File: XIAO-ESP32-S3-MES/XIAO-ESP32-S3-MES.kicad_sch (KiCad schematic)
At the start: 11 parts, among them J1 Conn_01x04_Socket, J2 Conn_01x02_Socket, J3 Conn_01x04_Socket, U2 XIAO-ESP32-S3-SMD

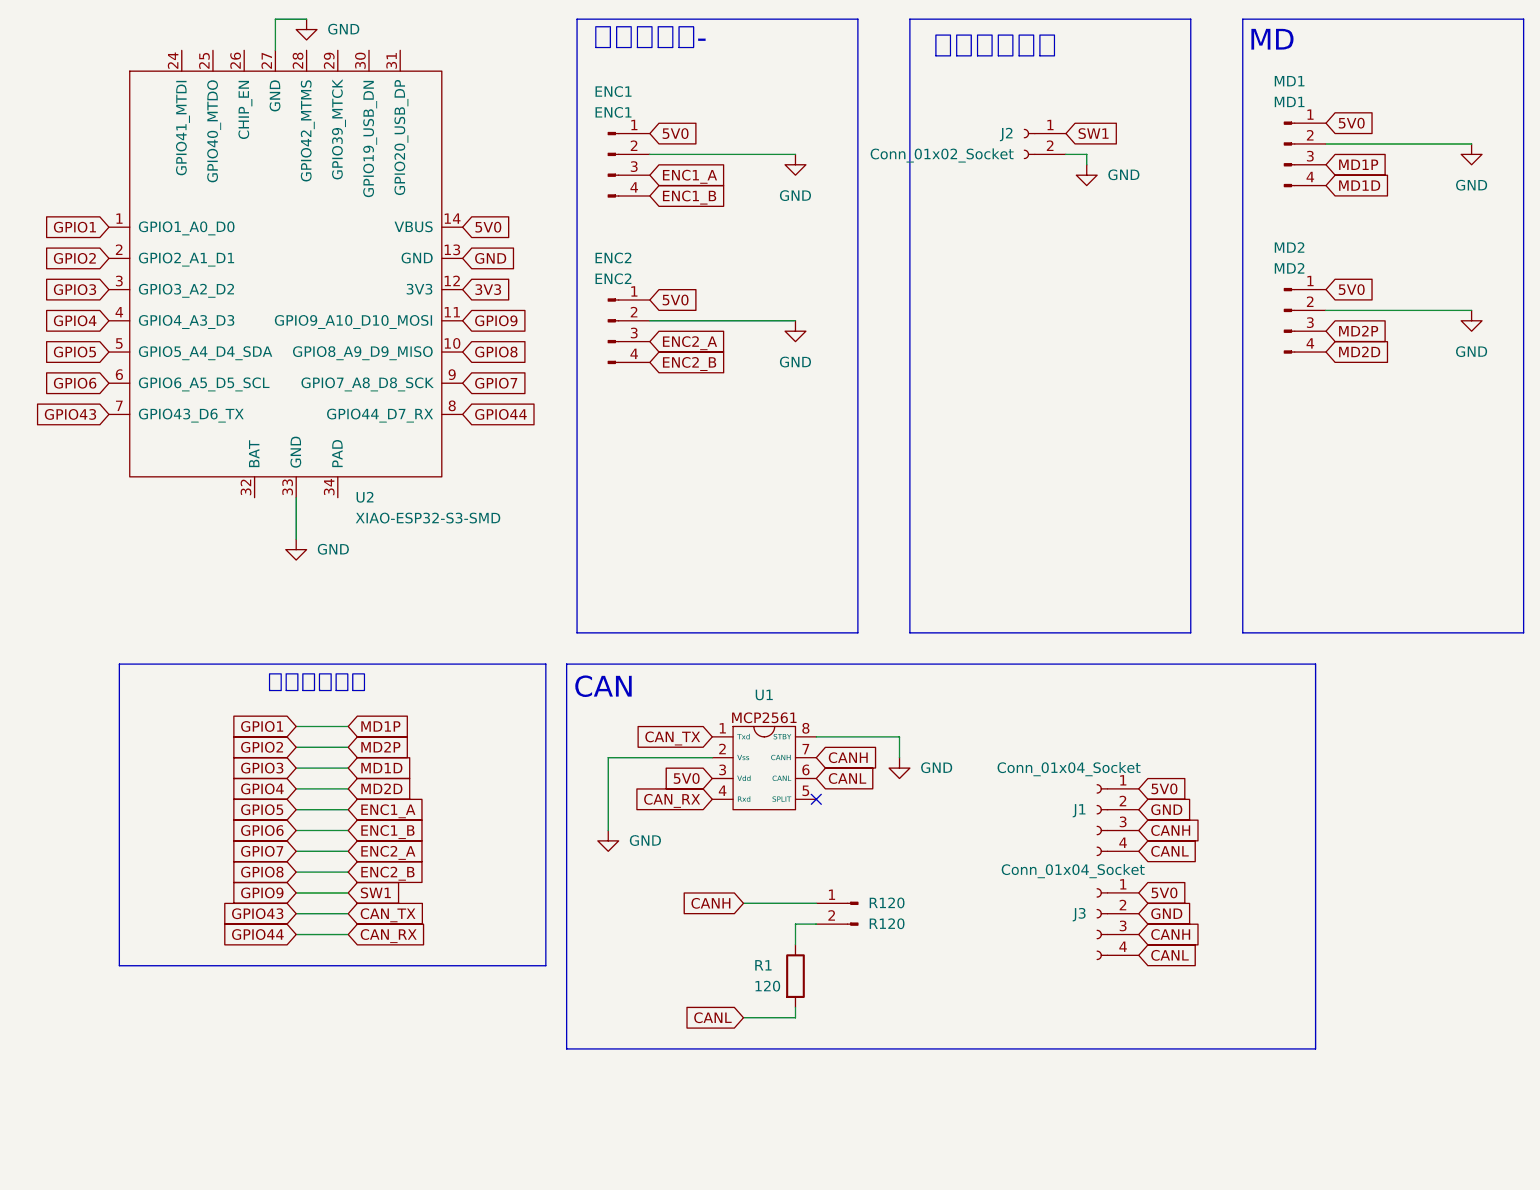
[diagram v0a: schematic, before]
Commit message: 汎用性重視
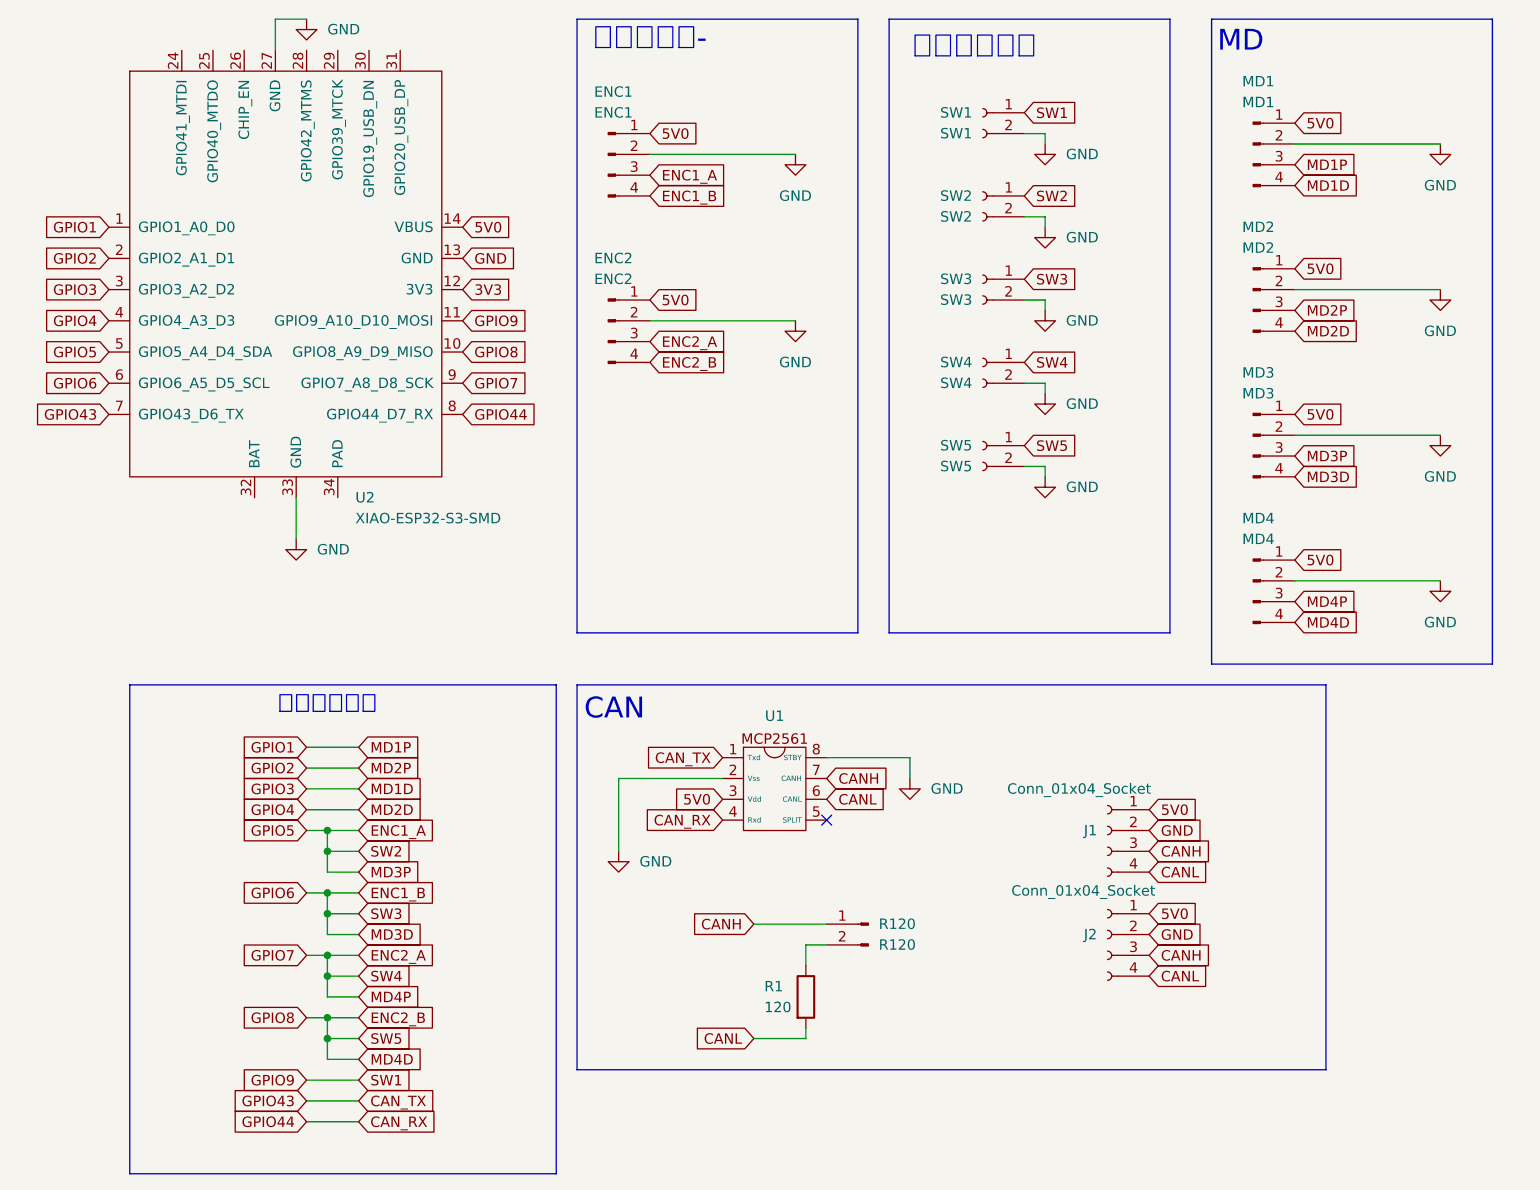
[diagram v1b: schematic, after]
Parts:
- added MD3: MD3, Connector_JST:JST_XH_B4B-XH-A_1x04_P2.50mm_Vertical, symbol Connector:Conn_01x04_Pin
- added MD4: MD4, Connector_JST:JST_XH_B4B-XH-A_1x04_P2.50mm_Vertical, symbol Connector:Conn_01x04_Pin
- added SW2: SW2, Connector_JST:JST_XH_B2B-XH-A_1x02_P2.50mm_Vertical, symbol Connector:Conn_01x02_Socket
- added SW3: SW3, Connector_JST:JST_XH_B2B-XH-A_1x02_P2.50mm_Vertical, symbol Connector:Conn_01x02_Socket
- added SW4: SW4, Connector_JST:JST_XH_B2B-XH-A_1x02_P2.50mm_Vertical, symbol Connector:Conn_01x02_Socket
- added SW5: SW5, Connector_JST:JST_XH_B2B-XH-A_1x02_P2.50mm_Vertical, symbol Connector:Conn_01x02_Socket
- SW1: renamed from J2; value Conn_01x02_Socket -> SW1
- renumbered J3 to J2
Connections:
- net 5V0: now also MD3.1 (Pin_1), MD4.1 (Pin_1)
- net ENC1_A: now also MD3.3 (Pin_3), SW2.1 (Pin_1)
- net ENC1_B: now also MD3.4 (Pin_4), SW3.1 (Pin_1)
- net ENC2_A: now also MD4.3 (Pin_3), SW4.1 (Pin_1)
- net ENC2_B: now also MD4.4 (Pin_4), SW5.1 (Pin_1)
- net GND: now also MD3.2 (Pin_2), MD4.2 (Pin_2), SW2.2 (Pin_2), SW3.2 (Pin_2), SW4.2 (Pin_2), SW5.2 (Pin_2)
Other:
- moved on the sheet: J1, J2, MD1, MD2, R1, R120, SW1, U1
